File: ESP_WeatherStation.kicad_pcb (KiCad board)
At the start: 2 copper layers, 23.7 x 38 mm, 19 parts, among them J1 Con1, U1 AZ1117-3.3, U2 ESP-12F, U3 Si7021, U4 BMP280, U5 DS1821C

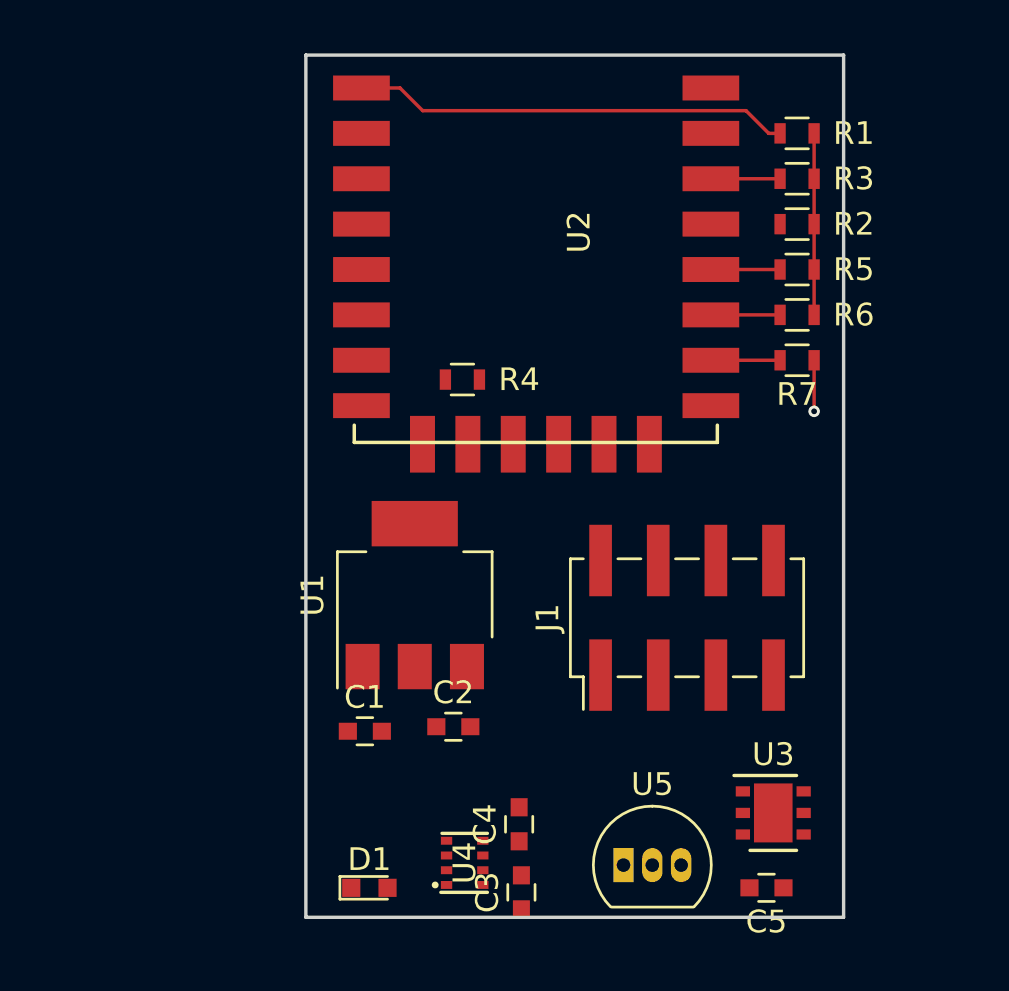
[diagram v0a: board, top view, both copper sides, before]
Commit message: Final version
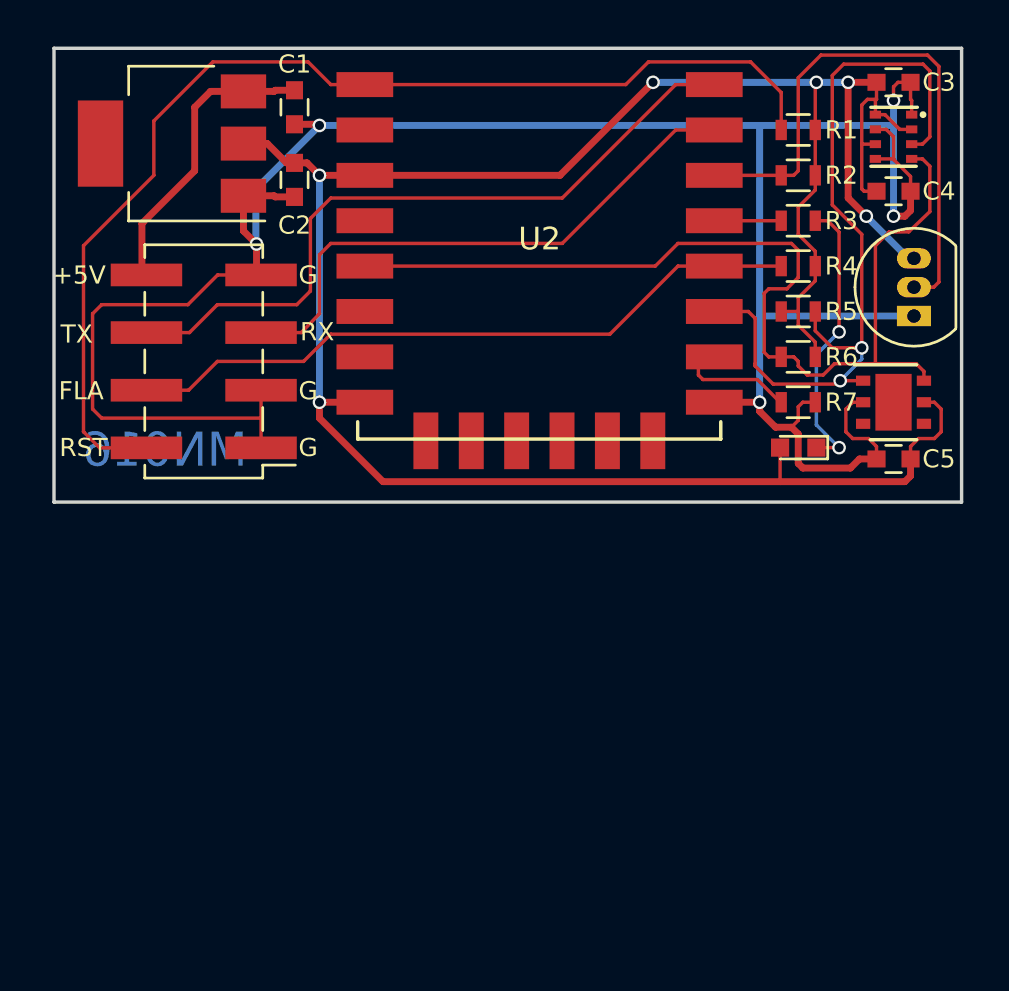
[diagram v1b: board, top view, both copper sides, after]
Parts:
- removed the R7 at (169.8, 117.8)
- added R6: 10k, Resistors_SMD:R_0603, F.Cu at (169.8, 117.6)
- R2: value 10k -> 4.7k
- R3: value 4.7k -> 82
- R4: value 82 -> 1k
- R5: value 1k -> 10k
- moved C3 39.3 mm to (174.0, 105.5), turned to 0 degrees
- moved U4 37.2 mm to (174.0, 107.9), turned to 270 degrees
- moved C4 32.4 mm to (174.0, 110.3), turned to 0 degrees
- moved C1 27.7 mm to (147.6, 106.6), turned to 270 degrees
- moved U5 27.4 mm to (174.9, 115.8), turned to 90 degrees
- moved D1 27.1 mm to (169.8, 121.6), turned to 180 degrees
- moved C2 25.1 mm to (147.6, 109.8), turned to 270 degrees
- moved J1 24.1 mm to (143.6, 117.8), turned to 180 degrees
- moved U1 22.6 mm to (142.2, 108.2), turned to 180 degrees
- moved C5 19.7 mm to (174.0, 122.1)
- moved U3 18.9 mm to (174.0, 119.6)
- moved R4 15.6 mm to (169.8, 113.6), turned to 180 degrees
- moved R7 3.85 mm to (169.8, 119.6)
- moved R2 2.15 mm to (169.8, 109.6), turned to 180 degrees
- moved R3 1.85 mm to (169.8, 111.6), turned to 0 degrees
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- renumbered R6 to R7
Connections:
- J1 pad 1: /RESET -> GND
- J1 pad 2: GND -> /RESET
- J1 pad 3: /BOOT -> GND
- J1 pad 4: GND -> /BOOT
- J1 pad 7: +5V -> GND
- J1 pad 8: GND -> +5V
- R2 pad 1: /SCL -> +3V3
- R2 pad 2: +3V3 -> /DATA
- R3 pad 1: +3V3 -> /LED
- R3 pad 2: /DATA -> Net-(D1-Pad1)
- R4 pad 1: /LED -> +3V3
- R4 pad 2: Net-(D1-Pad1) -> /BOOT
- R5 pad 2: /BOOT -> /SDA
- R7 pad 1: +3V3 -> GND
- R7 pad 2: /SDA -> Net-(R6-Pad2)
- U2 pad 10: Net-(R7-Pad2) -> Net-(R6-Pad2)
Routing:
- net GND: track 2.25 -> 110.6 mm, vias 1 -> 5
- net +3V3: track 8.00 -> 109.8 mm, vias 0 -> 6
- net /SCL: track 0.00 -> 44.0 mm
- net /SDA: track 3.75 -> 35.9 mm, vias 0 -> 2
- net /TXD: track 0.00 -> 31.0 mm
- net /RESET: track 18.6 -> 49.5 mm
- net /BOOT: track 3.75 -> 30.5 mm
- net /RXD: track 0.00 -> 24.8 mm
- net /DATA: track 3.75 -> 26.1 mm
- net +5V: track 0.00 -> 13.3 mm
- net Net-(D1-Pad1): track 0.00 -> 12.6 mm, vias 0 -> 2
- net Net-(R6-Pad2): track 0.00 -> 4.95 mm
- net Net-(R7-Pad2): track 3.75 -> 0.00 mm
- net /LED: track 0.00 -> 3.65 mm
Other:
- board size 23.7 x 38 mm -> 40 x 20 mm
- net class Default: clearance 0.2 -> 0.1524; trace_width 0.25 -> 0.1524; via_dia 0.6 -> 0.508; via_drill 0.4 -> 0.254
- rule pad_to_mask_clearance: 0.2 -> 0.0508
- rule trace_clearance: 0.2 -> 0.1524
- board text added: "(c)2018 MaxNil"
- board text added: "+5V"
- board text added: "ESP8266 Temperature Humidity Pressure"
- board text added: "FLA"
- board text added: "G"
- board text added: "MN016"
- board text added: "RST"
- board text added: "RX"
- board text added: "TX"
